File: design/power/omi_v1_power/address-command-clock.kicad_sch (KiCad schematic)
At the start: 9 parts

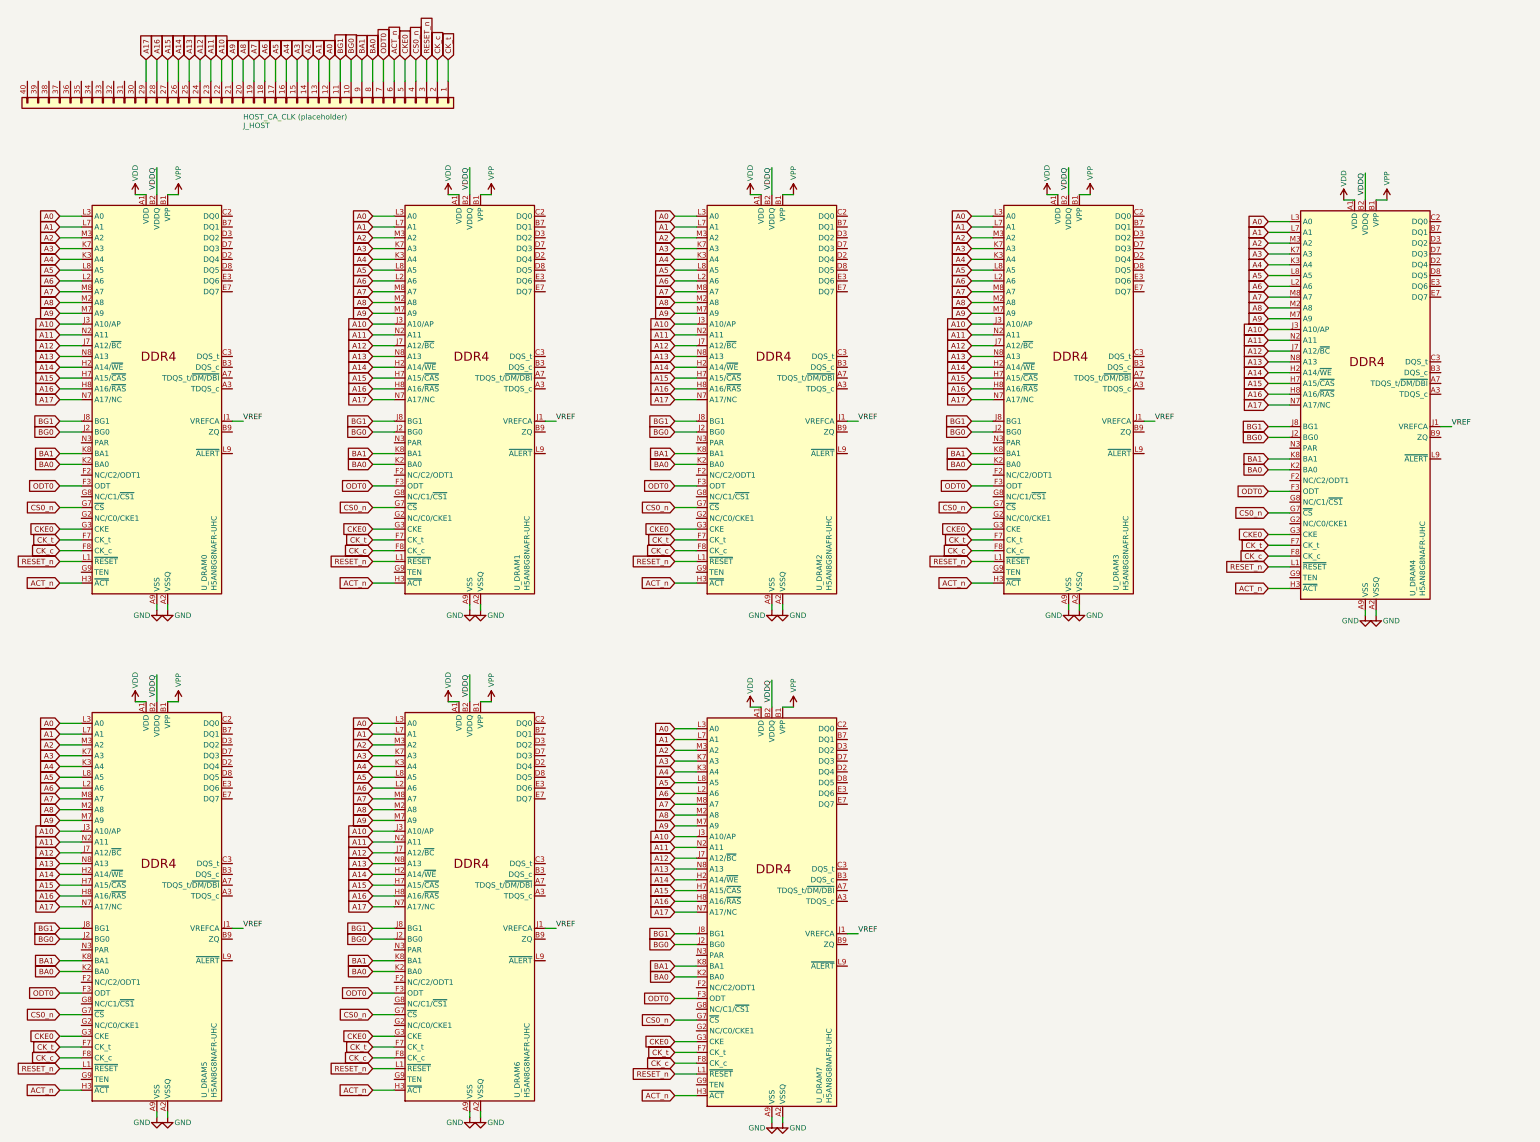
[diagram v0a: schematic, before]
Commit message: feat: Add OMI v1 Stage 7.3 DQ/DQS documentation and PDF artifact.
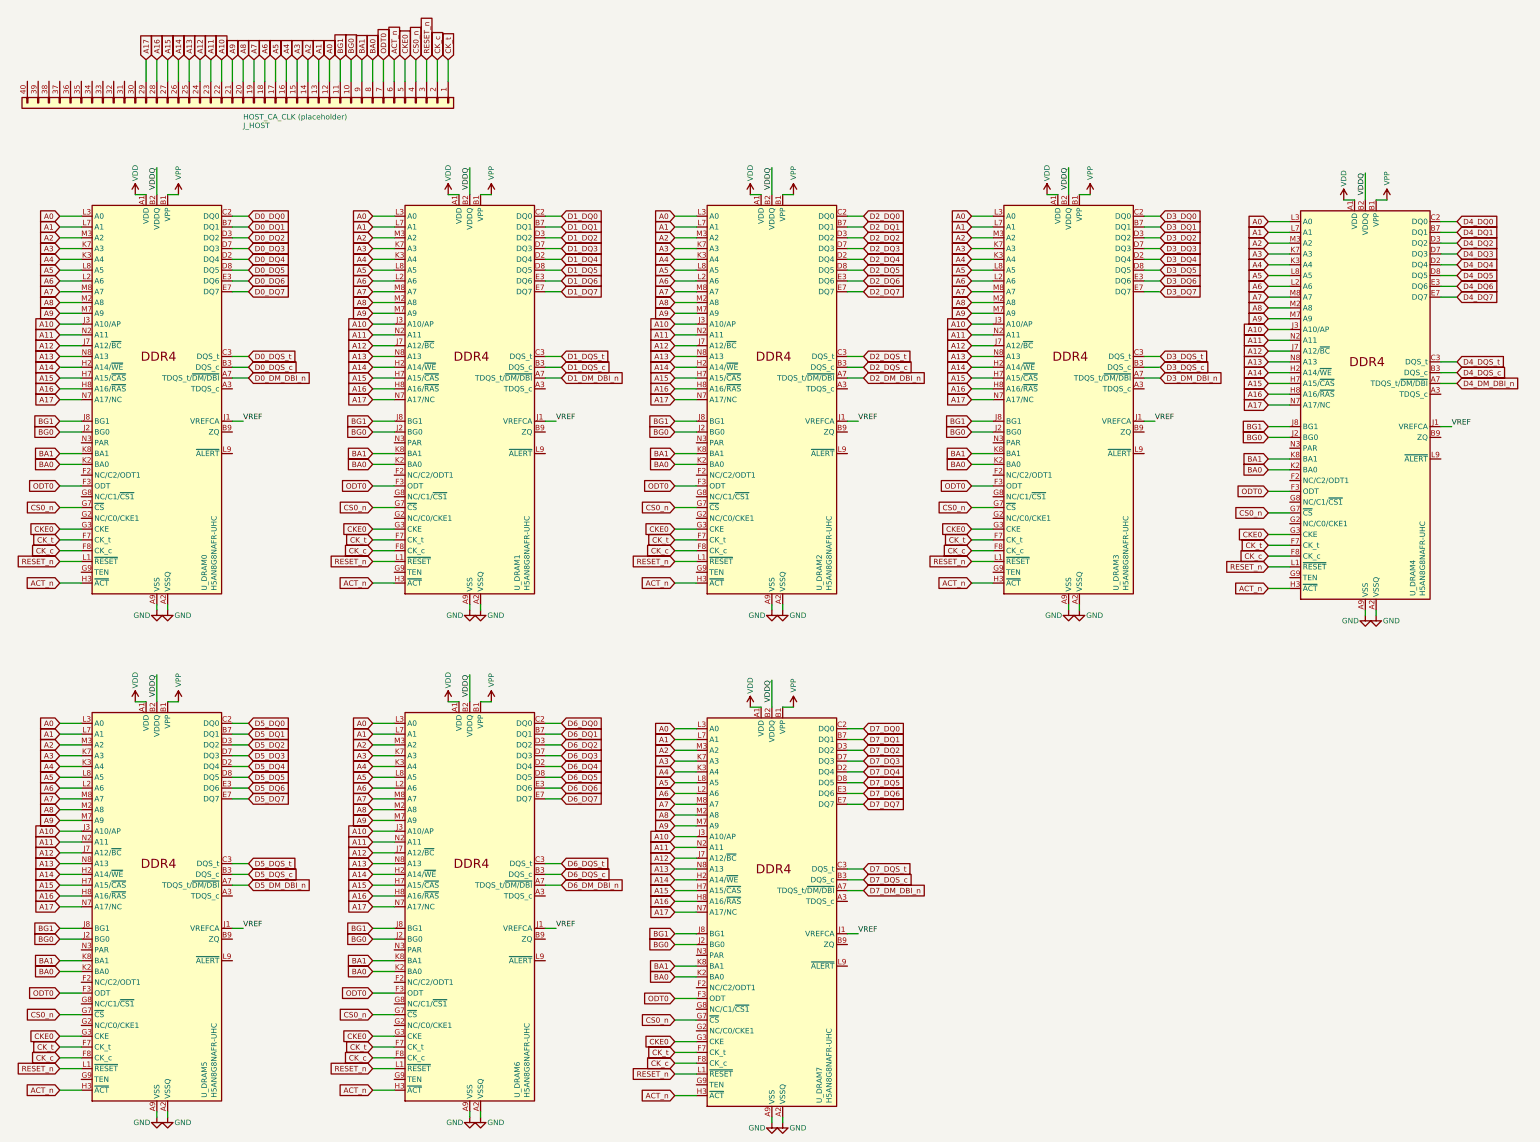
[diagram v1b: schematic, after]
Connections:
- net D7_DM_DBI_n: now reaches U_DRAM7.A7 (TDQS_t/~{DM/DBI})
- net D7_DQS_c: now reaches U_DRAM7.B3 (DQS_c)
- net D7_DQ1: now reaches U_DRAM7.B7 (DQ1)
- net D7_DQ0: now reaches U_DRAM7.C2 (DQ0)
- net D7_DQS_t: now reaches U_DRAM7.C3 (DQS_t)
- net D7_DQ4: now reaches U_DRAM7.D2 (DQ4)
- net D7_DQ2: now reaches U_DRAM7.D3 (DQ2)
- net D7_DQ3: now reaches U_DRAM7.D7 (DQ3)
- net D7_DQ5: now reaches U_DRAM7.D8 (DQ5)
- net D7_DQ6: now reaches U_DRAM7.E3 (DQ6)
- net D7_DQ7: now reaches U_DRAM7.E7 (DQ7)
- net D3_DM_DBI_n: now reaches U_DRAM3.A7 (TDQS_t/~{DM/DBI})
- net D3_DQS_c: now reaches U_DRAM3.B3 (DQS_c)
- net D3_DQ1: now reaches U_DRAM3.B7 (DQ1)
- net D3_DQ0: now reaches U_DRAM3.C2 (DQ0)
- net D3_DQS_t: now reaches U_DRAM3.C3 (DQS_t)
- net D3_DQ4: now reaches U_DRAM3.D2 (DQ4)
- net D3_DQ2: now reaches U_DRAM3.D3 (DQ2)
- net D3_DQ3: now reaches U_DRAM3.D7 (DQ3)
- net D3_DQ5: now reaches U_DRAM3.D8 (DQ5)
- net D3_DQ6: now reaches U_DRAM3.E3 (DQ6)
- net D3_DQ7: now reaches U_DRAM3.E7 (DQ7)
- net D2_DM_DBI_n: now reaches U_DRAM2.A7 (TDQS_t/~{DM/DBI})
- net D2_DQS_c: now reaches U_DRAM2.B3 (DQS_c)
- net D2_DQ1: now reaches U_DRAM2.B7 (DQ1)
- net D2_DQ0: now reaches U_DRAM2.C2 (DQ0)
- net D2_DQS_t: now reaches U_DRAM2.C3 (DQS_t)
- net D2_DQ4: now reaches U_DRAM2.D2 (DQ4)
- net D2_DQ2: now reaches U_DRAM2.D3 (DQ2)
- net D2_DQ3: now reaches U_DRAM2.D7 (DQ3)
- net D2_DQ5: now reaches U_DRAM2.D8 (DQ5)
- net D2_DQ6: now reaches U_DRAM2.E3 (DQ6)
- net D2_DQ7: now reaches U_DRAM2.E7 (DQ7)
- net D4_DM_DBI_n: now reaches U_DRAM4.A7 (TDQS_t/~{DM/DBI})
- net D4_DQS_c: now reaches U_DRAM4.B3 (DQS_c)
- net D4_DQ1: now reaches U_DRAM4.B7 (DQ1)
- net D4_DQ0: now reaches U_DRAM4.C2 (DQ0)
- net D4_DQS_t: now reaches U_DRAM4.C3 (DQS_t)
- net D4_DQ4: now reaches U_DRAM4.D2 (DQ4)
- net D4_DQ2: now reaches U_DRAM4.D3 (DQ2)
- net D4_DQ3: now reaches U_DRAM4.D7 (DQ3)
- net D4_DQ5: now reaches U_DRAM4.D8 (DQ5)
- net D4_DQ6: now reaches U_DRAM4.E3 (DQ6)
- net D4_DQ7: now reaches U_DRAM4.E7 (DQ7)
- net D5_DM_DBI_n: now reaches U_DRAM5.A7 (TDQS_t/~{DM/DBI})
- net D5_DQS_c: now reaches U_DRAM5.B3 (DQS_c)
- net D5_DQ1: now reaches U_DRAM5.B7 (DQ1)
- net D5_DQ0: now reaches U_DRAM5.C2 (DQ0)
- net D5_DQS_t: now reaches U_DRAM5.C3 (DQS_t)
- net D5_DQ4: now reaches U_DRAM5.D2 (DQ4)
- net D5_DQ2: now reaches U_DRAM5.D3 (DQ2)
- net D5_DQ3: now reaches U_DRAM5.D7 (DQ3)
- net D5_DQ5: now reaches U_DRAM5.D8 (DQ5)
- net D5_DQ6: now reaches U_DRAM5.E3 (DQ6)
- net D5_DQ7: now reaches U_DRAM5.E7 (DQ7)
- net D1_DM_DBI_n: now reaches U_DRAM1.A7 (TDQS_t/~{DM/DBI})
- net D1_DQS_c: now reaches U_DRAM1.B3 (DQS_c)
- net D1_DQ1: now reaches U_DRAM1.B7 (DQ1)
- net D1_DQ0: now reaches U_DRAM1.C2 (DQ0)
- net D1_DQS_t: now reaches U_DRAM1.C3 (DQS_t)
- net D1_DQ4: now reaches U_DRAM1.D2 (DQ4)
- net D1_DQ2: now reaches U_DRAM1.D3 (DQ2)
- net D1_DQ3: now reaches U_DRAM1.D7 (DQ3)
- net D1_DQ5: now reaches U_DRAM1.D8 (DQ5)
- net D1_DQ6: now reaches U_DRAM1.E3 (DQ6)
- net D1_DQ7: now reaches U_DRAM1.E7 (DQ7)
- net D0_DM_DBI_n: now reaches U_DRAM0.A7 (TDQS_t/~{DM/DBI})
- net D0_DQS_c: now reaches U_DRAM0.B3 (DQS_c)
- net D0_DQ1: now reaches U_DRAM0.B7 (DQ1)
- net D0_DQ0: now reaches U_DRAM0.C2 (DQ0)
- net D0_DQS_t: now reaches U_DRAM0.C3 (DQS_t)
- net D0_DQ4: now reaches U_DRAM0.D2 (DQ4)
- net D0_DQ2: now reaches U_DRAM0.D3 (DQ2)
- net D0_DQ3: now reaches U_DRAM0.D7 (DQ3)
- net D0_DQ5: now reaches U_DRAM0.D8 (DQ5)
- net D0_DQ6: now reaches U_DRAM0.E3 (DQ6)
- net D0_DQ7: now reaches U_DRAM0.E7 (DQ7)
- net D6_DM_DBI_n: now reaches U_DRAM6.A7 (TDQS_t/~{DM/DBI})
- net D6_DQS_c: now reaches U_DRAM6.B3 (DQS_c)
- net D6_DQ1: now reaches U_DRAM6.B7 (DQ1)
- net D6_DQ0: now reaches U_DRAM6.C2 (DQ0)
- net D6_DQS_t: now reaches U_DRAM6.C3 (DQS_t)
- net D6_DQ4: now reaches U_DRAM6.D2 (DQ4)
- net D6_DQ2: now reaches U_DRAM6.D3 (DQ2)
- net D6_DQ3: now reaches U_DRAM6.D7 (DQ3)
- net D6_DQ5: now reaches U_DRAM6.D8 (DQ5)
- net D6_DQ6: now reaches U_DRAM6.E3 (DQ6)
- net D6_DQ7: now reaches U_DRAM6.E7 (DQ7)
